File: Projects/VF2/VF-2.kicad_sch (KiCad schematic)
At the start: 39 parts, among them P1 2k2, T1 MPSA42, T2 MPSA93, T3 IRF9540, T4 IRF540, U1 Opa2134, U2 OPA2134

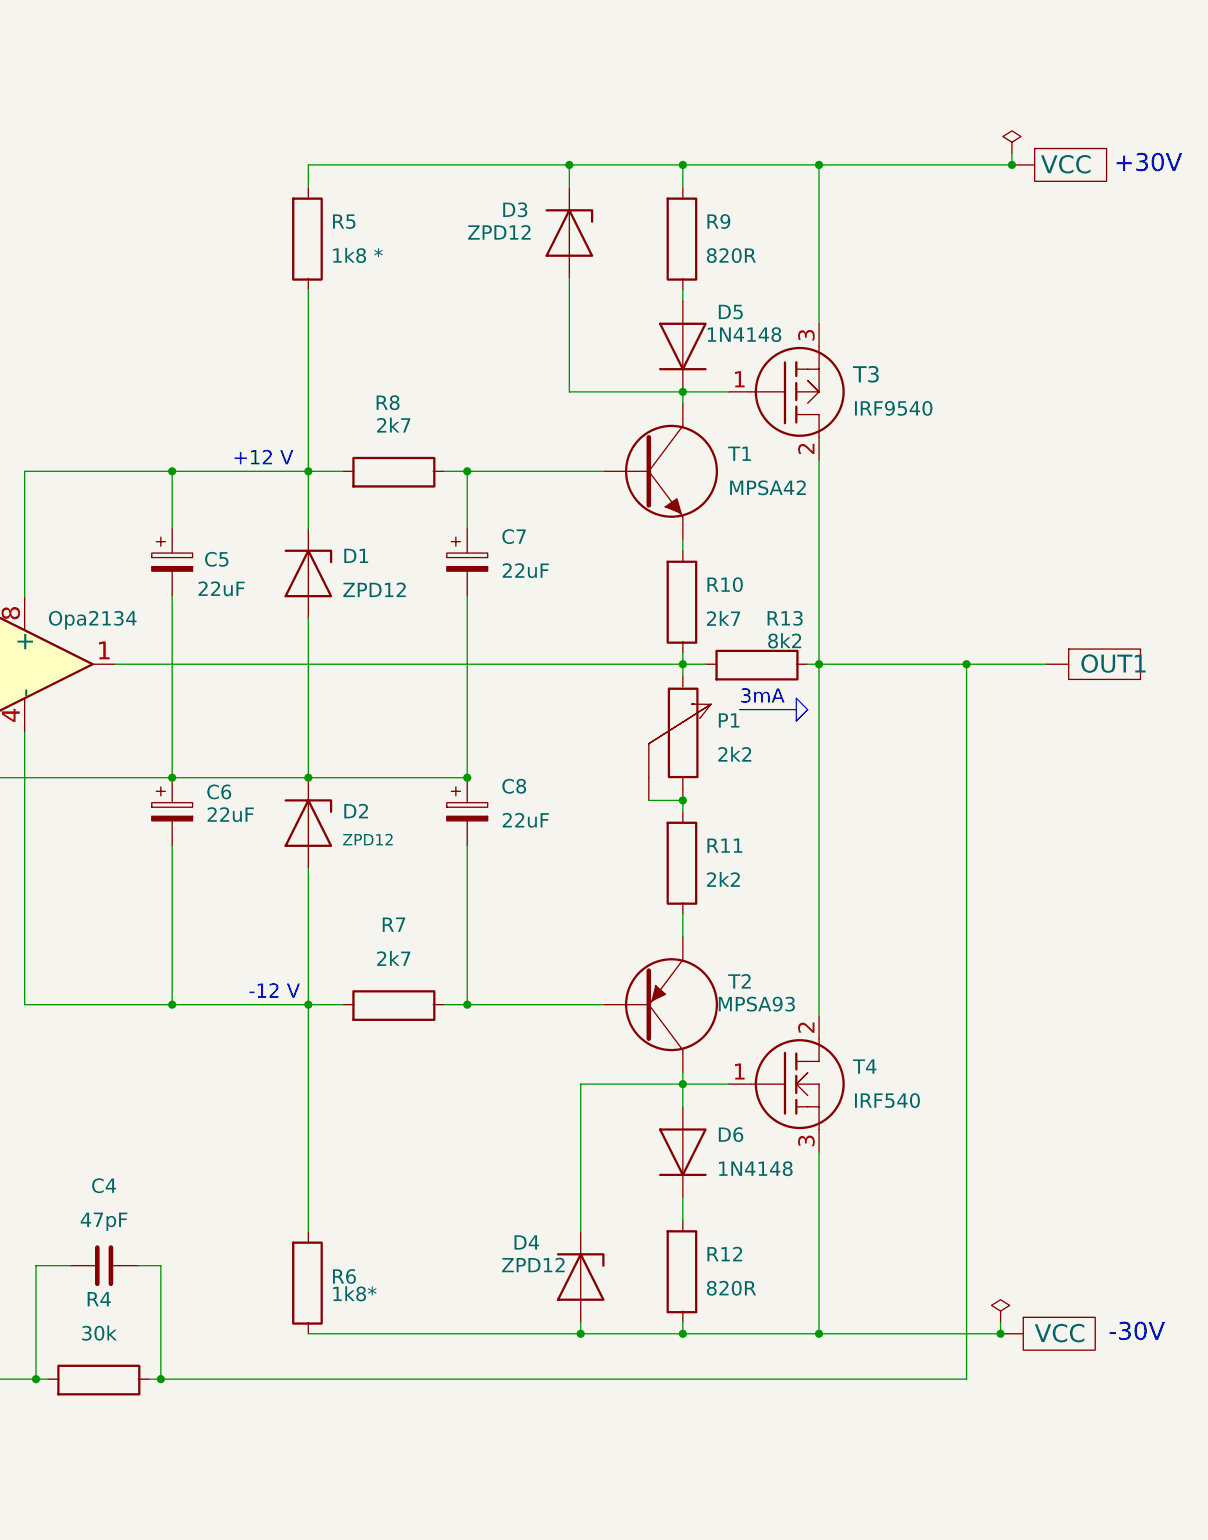
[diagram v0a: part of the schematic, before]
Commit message: 2
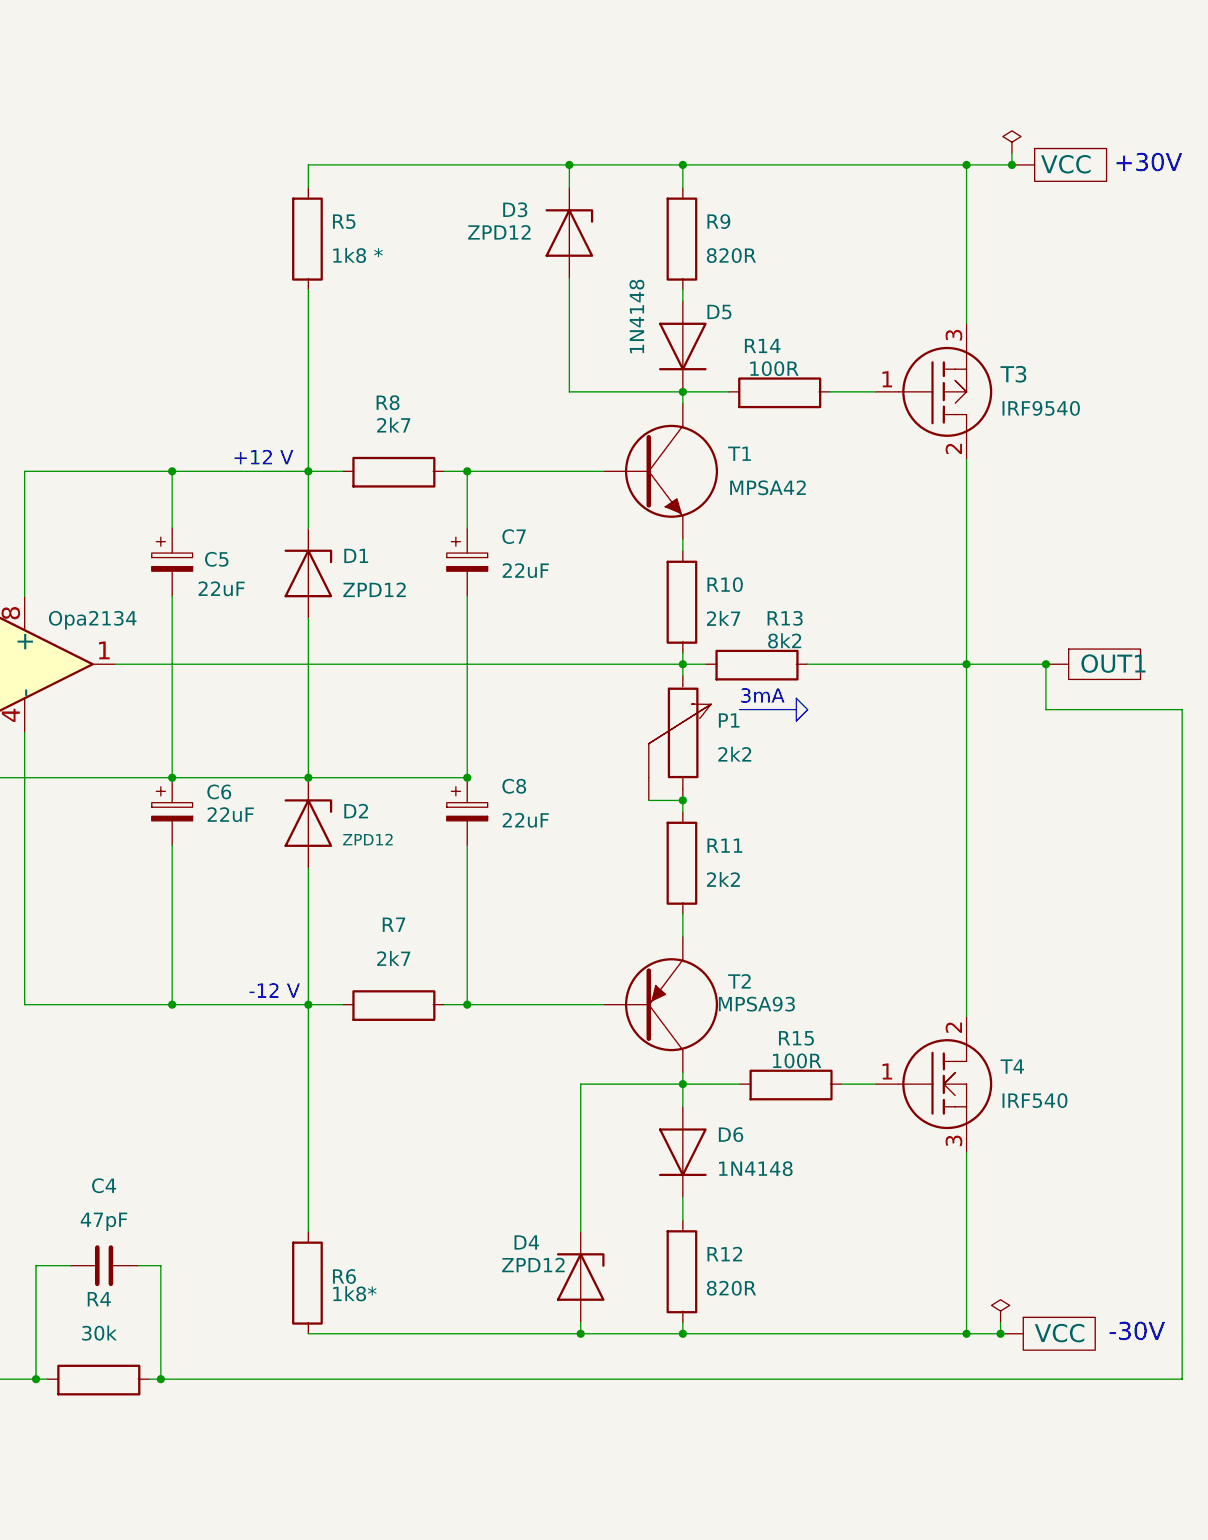
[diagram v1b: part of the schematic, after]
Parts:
- added R14, R15: 100R, symbol 000_Device:R
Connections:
- net at D3.2 (A), D5.1 (K), T1. (E): now also R14.2; no longer T3.1 (G)
- net at D4.1 (K), D6.2 (A), T2. (E): now also R15.2; no longer T4.1 (G)
- new net: R15.1, T4.1 (G)
- new net: R14.1, T3.1 (G)
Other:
- moved on the sheet: T3, T4

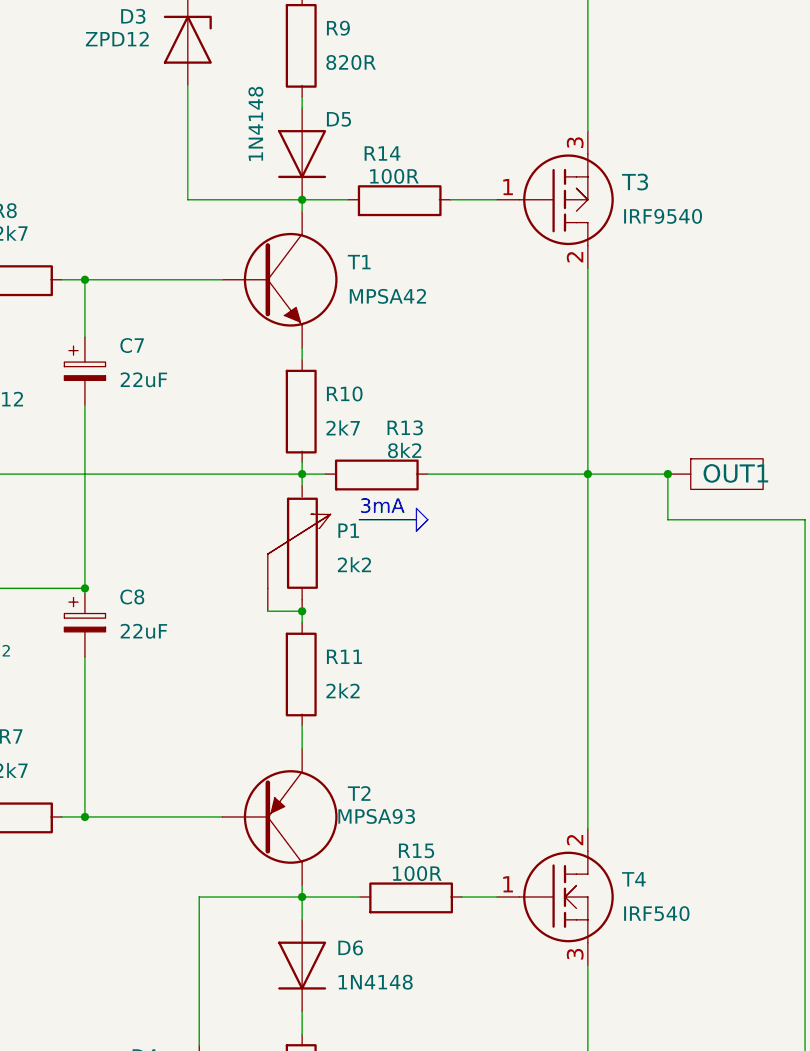
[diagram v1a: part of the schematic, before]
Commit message: 1
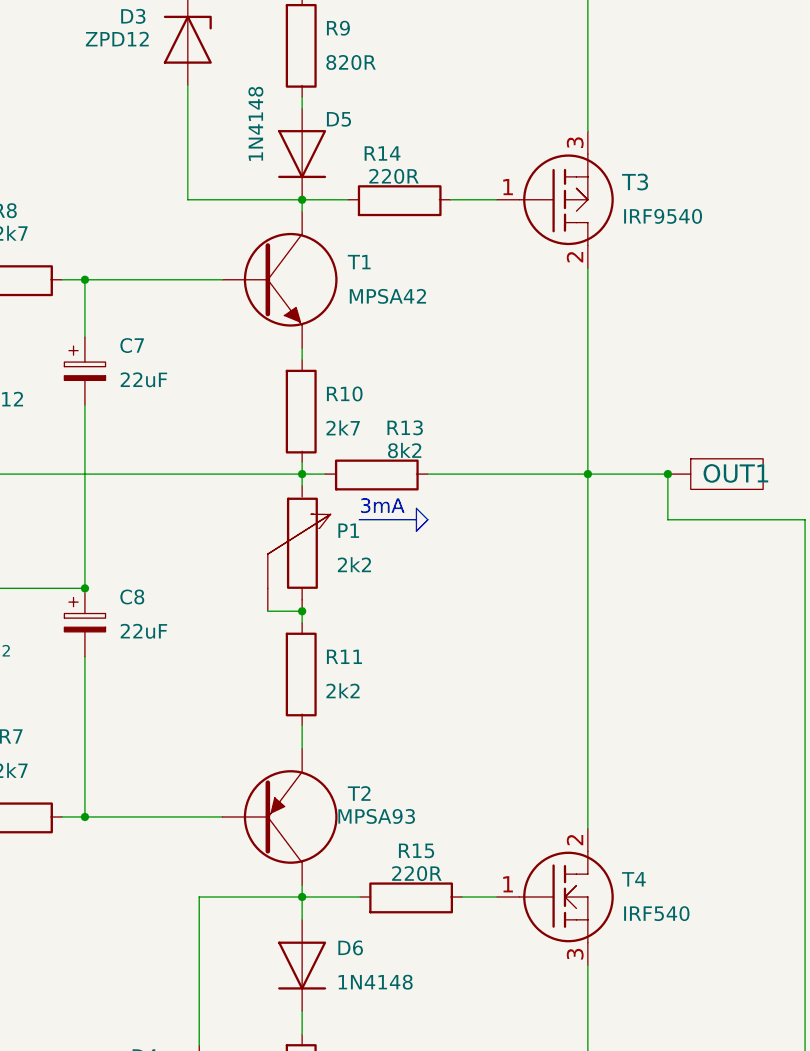
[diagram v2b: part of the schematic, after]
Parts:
- R14, R15: value 100R -> 220R
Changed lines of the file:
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@@
 			)
 		)
-		(property "Value" "100R"
+		(property "Value" "220R"
 			(at 196.85 138.43 90)
 			(show_name no)
@@
 			)
 		)
-		(property "Value" "100R"
+		(property "Value" "220R"
 			(at 194.31 60.96 90)
 			(show_name no)

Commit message: 2
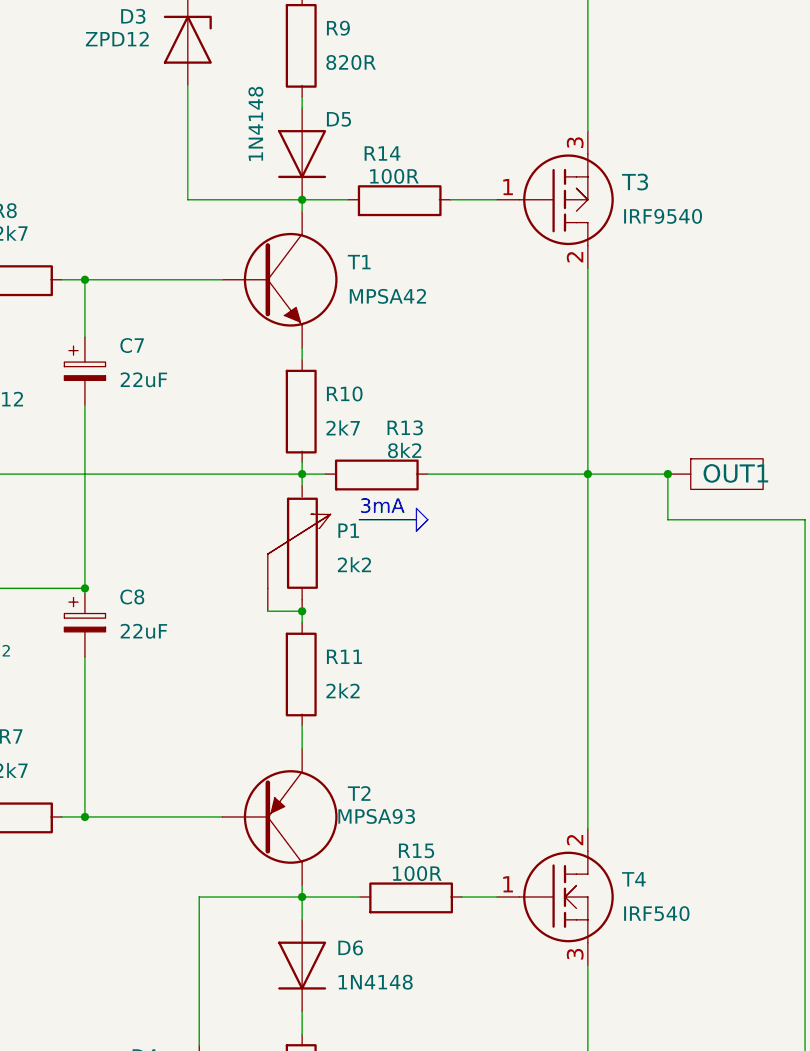
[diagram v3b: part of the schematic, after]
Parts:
- R14, R15: value 220R -> 100R
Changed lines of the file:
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@@
 			)
 		)
-		(property "Value" "220R"
+		(property "Value" "100R"
 			(at 196.85 138.43 90)
 			(show_name no)
@@
 			)
 		)
-		(property "Value" "220R"
+		(property "Value" "100R"
 			(at 194.31 60.96 90)
 			(show_name no)
